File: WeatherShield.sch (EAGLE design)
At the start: 66 parts, among them J7 M023.5MM, J8 M023.5MM, Q1 BSS138, Q2 BSS138, U1 DS3231SN, U2 LT3652, U4 MPL3115A2LGA8, U5 HTU21D

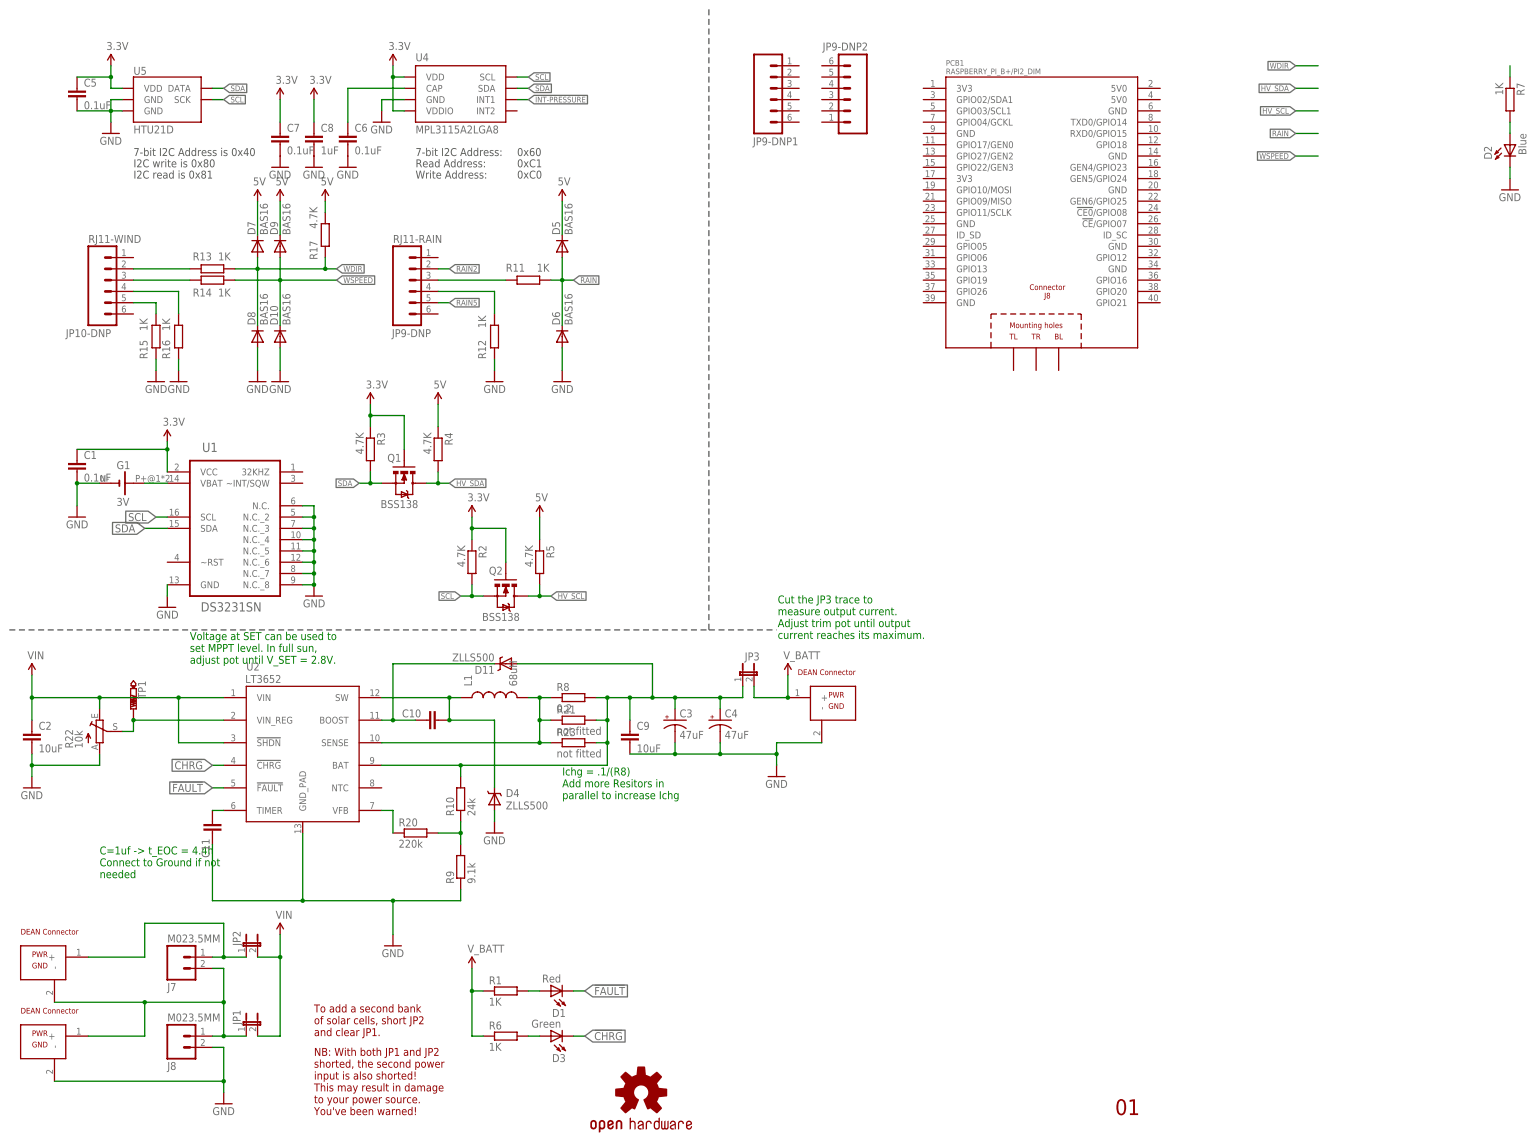
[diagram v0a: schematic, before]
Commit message: Power parts
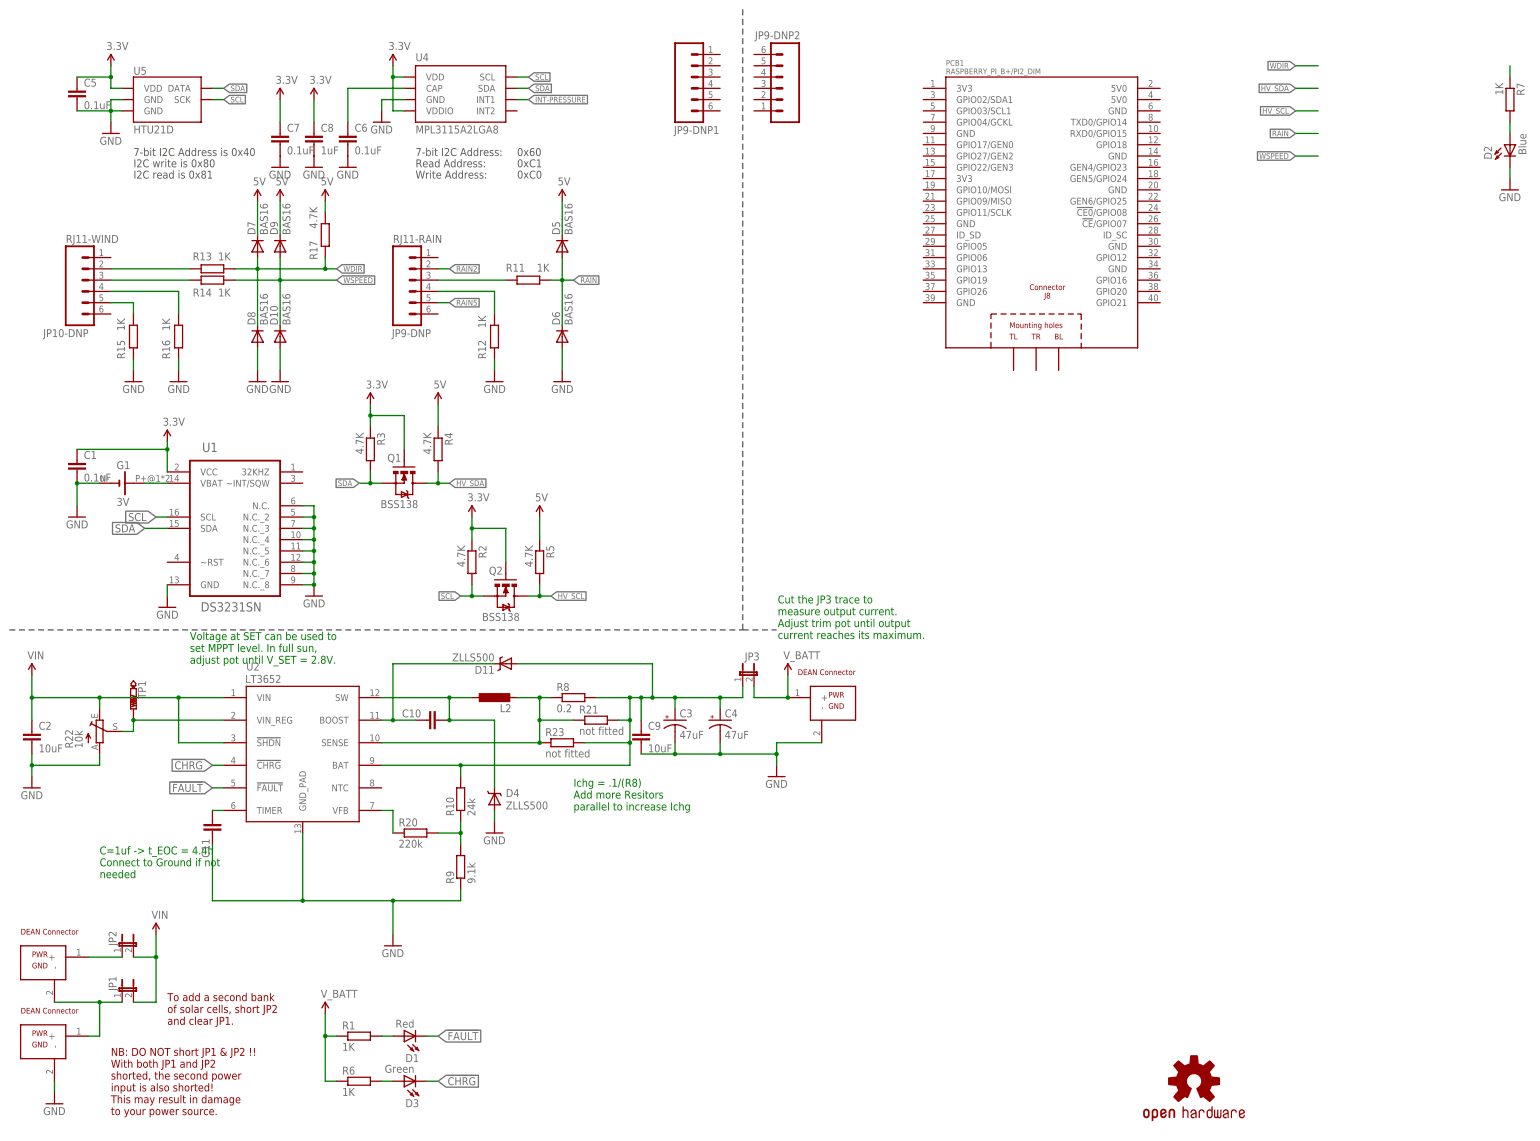
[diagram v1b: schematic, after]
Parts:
- removed J7, J8: M023.5MM, SparkFun-Connectors:M023.5MM
- removed L1: 68uH, SparkFun-Passives:INDUCTOR68UH-1A
- added L2: (no value), rcl:L-EU6000-XXX-RC
- C3, C4: device SparkFun-Capacitors:47UF-TANT -> FSEWeatherShield:47UF-16V-10%(TANT)
- R21, R23, R8: device rcl:R-EU_R0603 -> rcl:R-EU_R0805
- U$3: value DEAN_CONNECTOR -> V_BATT
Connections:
- net GND: no longer J8.2
- net N$14: no longer J7.2, J8.1
- net SENSE: now also L2.2; no longer L1.2
- net SFSASDF: no longer J7.1
- net SW: now also L2.1; no longer L1.1
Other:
- note added: "Ichg = .1/(R8) Add more Resitors parallel to increase Ichg"
- note added: "NB: DO NOT short JP1 & JP2 !! With both JP1 and JP2 shorted, the second power input is also shorted! This may result in damage to your power source."
- note removed: "01"
- note removed: "Ichg = .1/(R8) Add more Resitors in parallel to increase Ichg"
- note removed: "NB: With both JP1 and JP2 shorted, the second power input is also shorted! This may result in damage to your power source. You've been warned!"
- moved on the sheet: C9, D1, D3, JP1, JP10-DNP, JP2, JP9-DNP1, JP9-DNP2, R1, R15, R21, R23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
